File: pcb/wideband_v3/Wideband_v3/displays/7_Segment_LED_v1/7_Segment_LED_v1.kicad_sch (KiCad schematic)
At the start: 13 parts, among them J1 Conn_01x10, Q1 BC847, U5 4511, U7 SM420561N

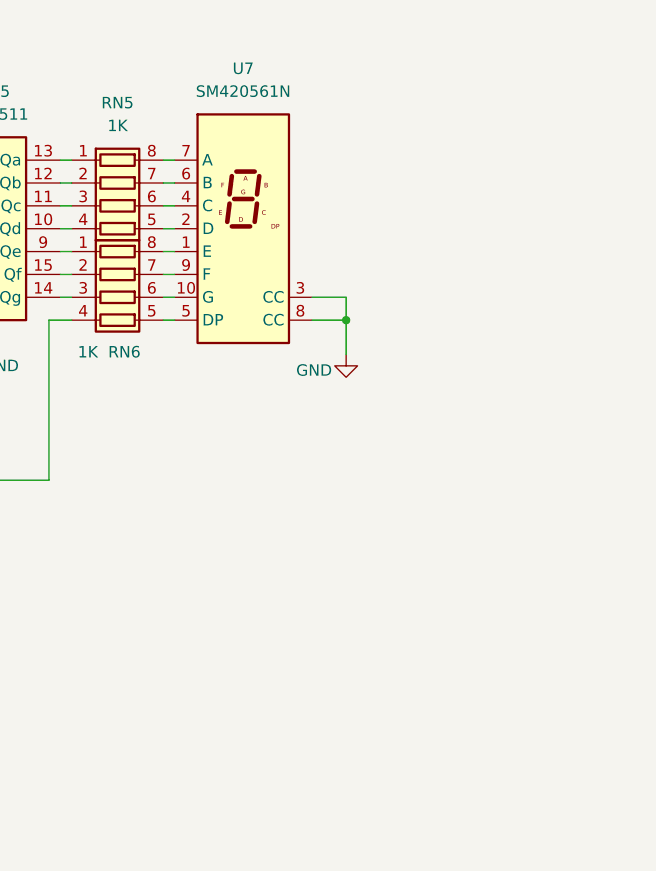
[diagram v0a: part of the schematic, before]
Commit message: update DAC for v3
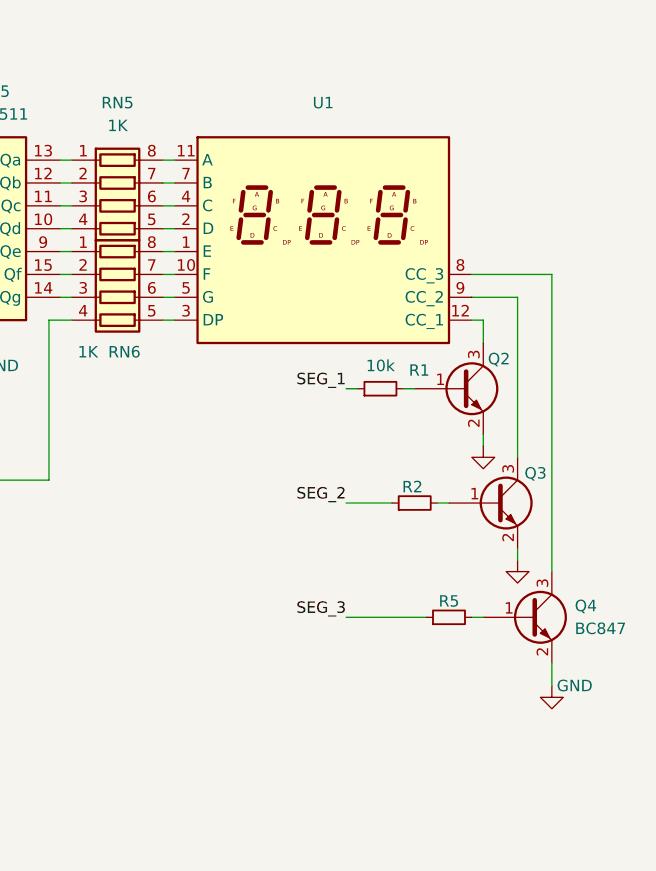
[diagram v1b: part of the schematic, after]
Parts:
- removed U7: SM420561N, Display_7Segment:SA15-11xxx, symbol Display_Character:SM420561N
- added Q2, Q3, Q4: BC847, Package_TO_SOT_THT:TO-92S_Wide, symbol Transistor_BJT:BC847
- added R1, R2, R5: 10k, Resistor_SMD:R_0603_1608Metric, symbol Device:R_Small
- added U1: ~, symbol New_Library:7seg_3digit
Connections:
- net GND: now also Q2.2 (E), Q3.2 (E), Q4.2 (E)
- net at RN6.8 (R1.2): now also U1.1 (E)
- net at RN6.6 (R3.2): now also U1.5 (G)
- net at RN5.5 (R4.2): now also U1.2 (D)
- net at RN5.6 (R3.2): now also U1.4 (C)
- net at RN6.5 (R4.2): now also U1.3 (DP)
- net at RN5.7 (R2.2): now also U1.7 (B)
- net at RN5.8 (R1.2): now also U1.11 (A)
- net at RN6.7 (R2.2): now also U1.10 (F)
- new net: Q2.3 (C), U1.12 (CC_1)
- new net: Q4.3 (C), U1.8 (CC_3)
- new net: Q3.3 (C), U1.9 (CC_2)
- new net: Q4.1 (B), R5.2
- new net: Q3.1 (B), R2.2
- new net: Q2.1 (B), R1.2
- new net SEG_1: R1.1
- new net SEG_2: R2.1
- new net SEG_3: R5.1
